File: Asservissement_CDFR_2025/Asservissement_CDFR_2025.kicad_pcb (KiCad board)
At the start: 4 copper layers, 90 x 90 mm, 196 parts, among them IC1 A3930KJPTR-T, IC2 A3930KJPTR-T, IC3 A3930KJPTR-T, J1 Connecteur batterie, J10 Conn_01x05, J11 Conn_01x03, J2 Conn_01x05, J3 Conn_01x03, J4 Connecteur Programmation, J5 Conn_01x03, J6 I2C_Master_Odo, J7 I2C_Slave, J8 Conn_01x05, J9 Conn_01x03, Q1 QM6006D, Q10 QM6006D, Q11 QM6006D, Q12 QM6006D, Q13 QM6006D, Q14 QM6006D, Q15 QM6006D, Q16 QM6006D, Q17 QM6006D, Q18 QM6006D, Q19 QM6006D, Q2 QM6006D, Q3 QM6006D, Q4 QM6006D, Q5 QM6006D, Q6 QM6006D, Q8 QM6006D, Q9 QM6006D, SW1 SW_Push, SW2 SW_Test, SW3 SW_Reset, U1 LMR16020PDDA, U2 LM317_SOT-223, U3 STM32F401RCTx

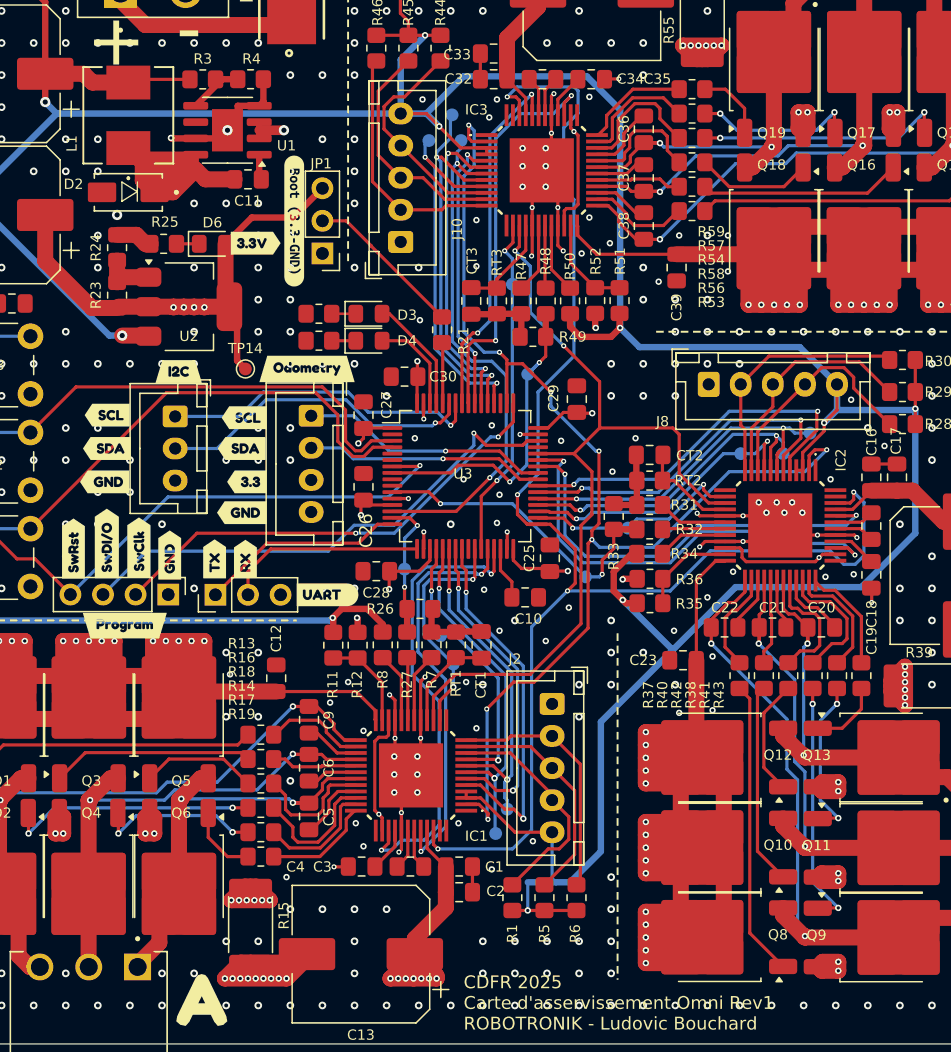
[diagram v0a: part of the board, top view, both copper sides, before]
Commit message: final
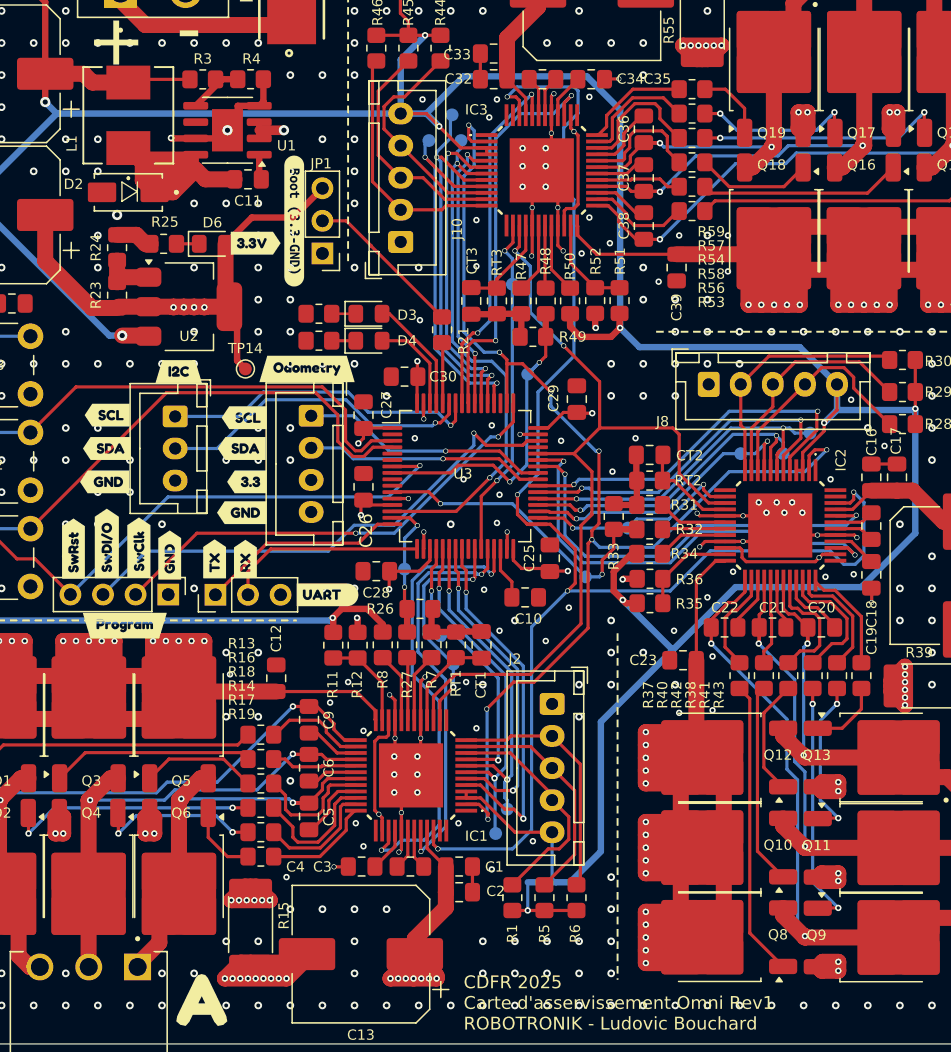
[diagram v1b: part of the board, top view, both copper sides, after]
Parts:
- F1: value 0154010.DR -> 0154010.DR
